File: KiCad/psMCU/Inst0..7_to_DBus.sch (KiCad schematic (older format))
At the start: 6 parts

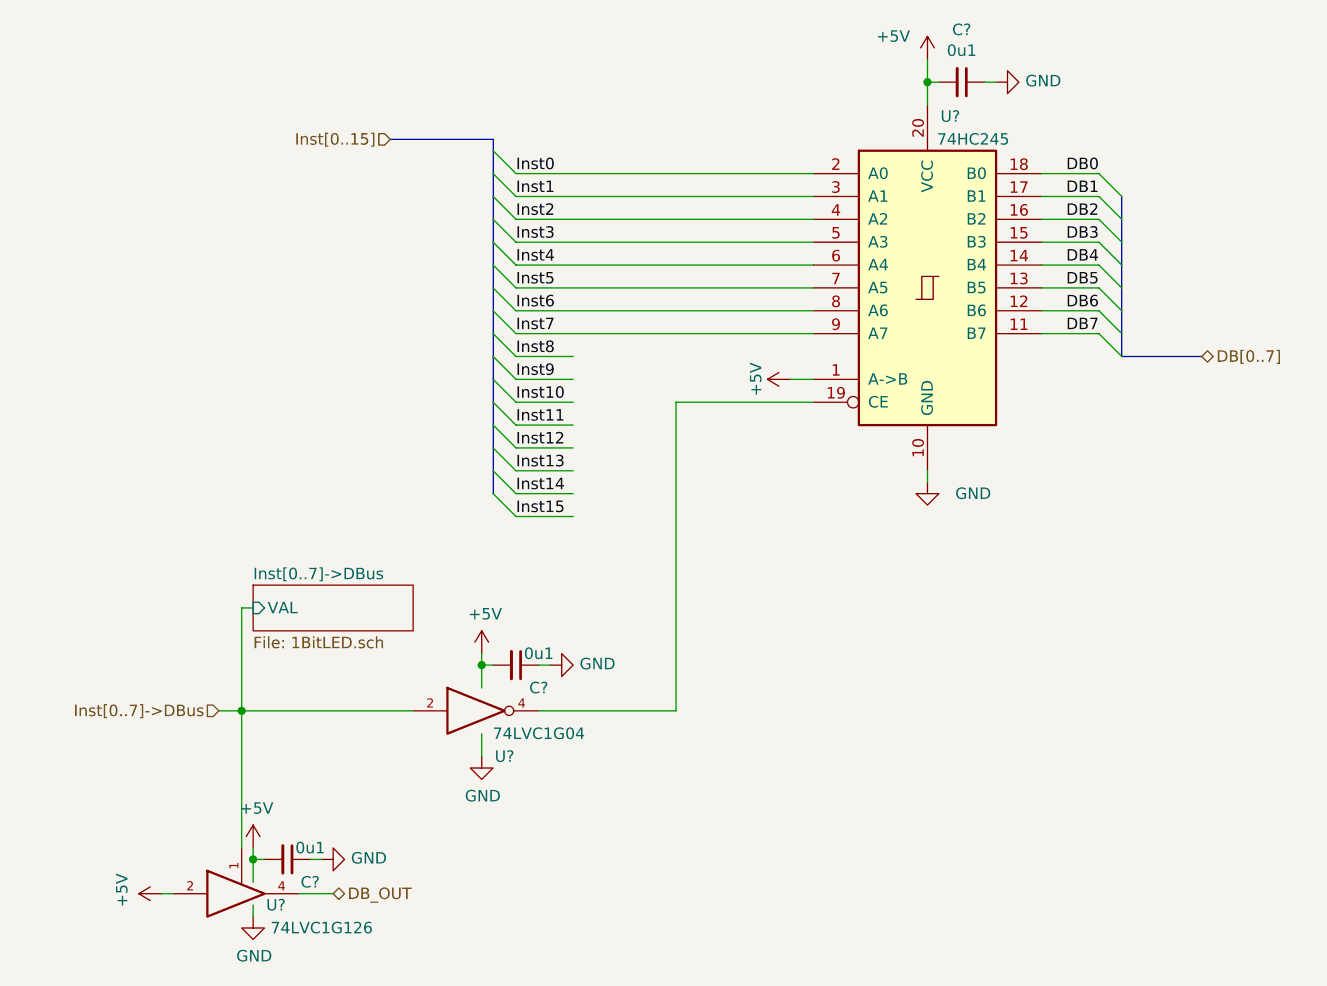
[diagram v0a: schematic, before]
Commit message: Started work on schematic
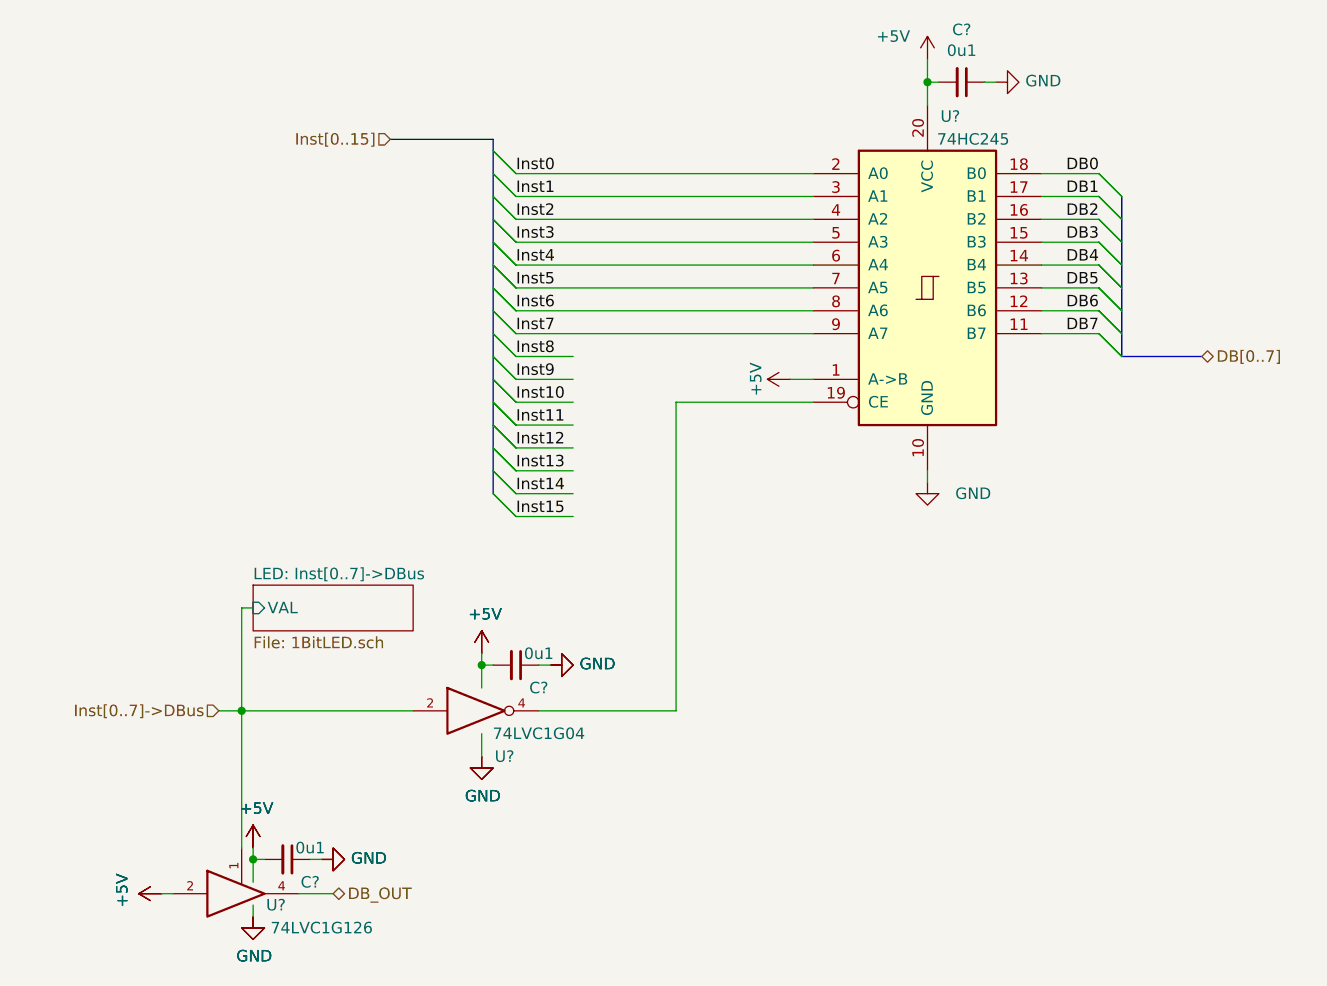
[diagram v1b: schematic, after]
